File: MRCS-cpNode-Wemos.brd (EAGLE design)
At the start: 99.8 x 68.8 mm, 40 parts, among them CON1 3.5MM, CON2 3.5MM, J2 CONNECTOR-GROVE-4P-2.0-347013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, Q2 2n7002, Q3 2n7002, Q4 2n7002, Q5 2n7002, U3 NE555P, U4 MAX3465CPD

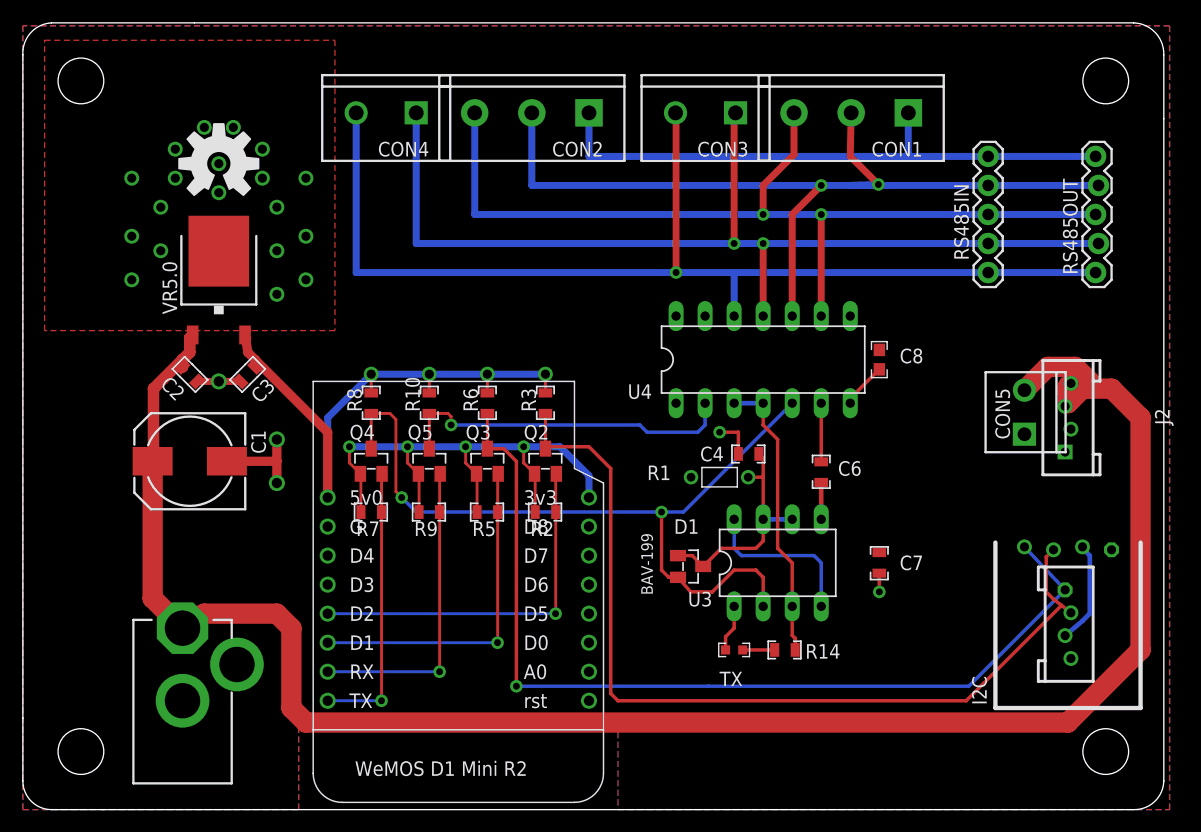
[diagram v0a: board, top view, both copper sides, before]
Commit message: 5.0
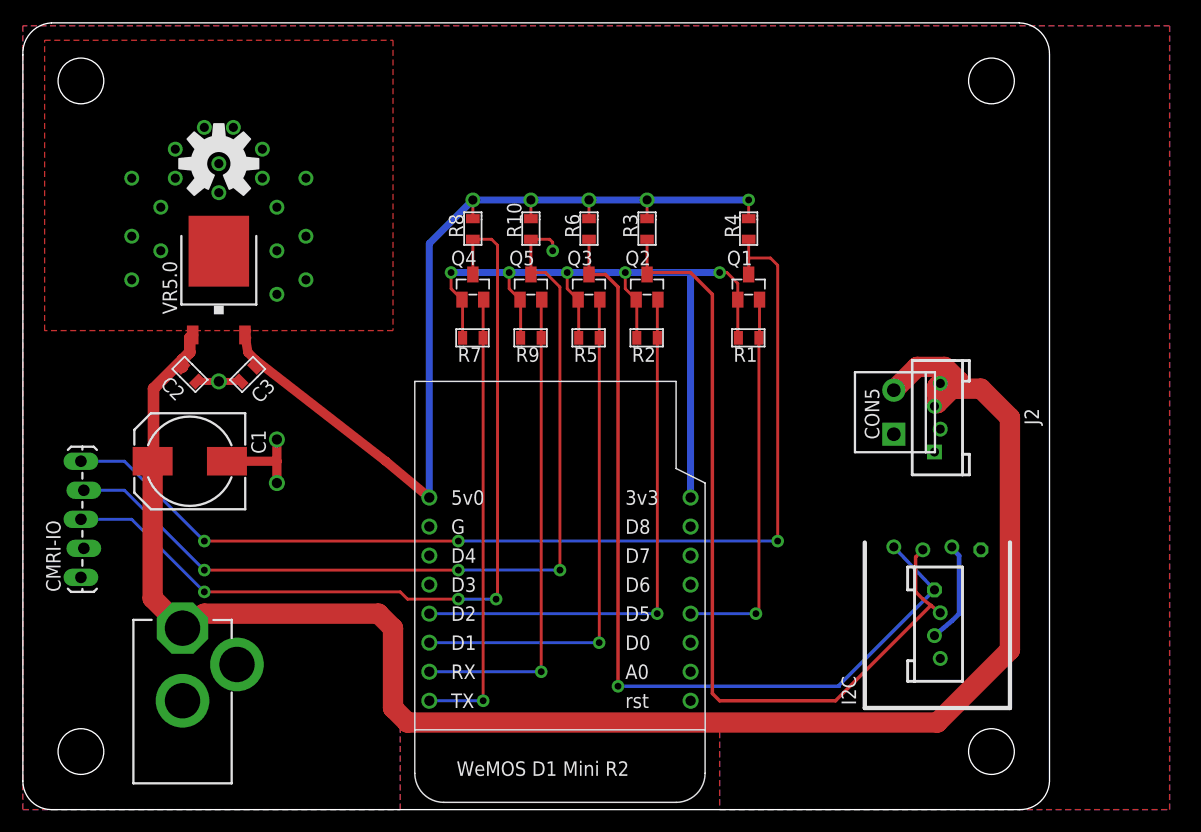
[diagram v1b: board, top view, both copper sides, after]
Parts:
- removed C4: 0.1uF, SPCoast:0805-CAP
- removed C6: .01uF, SPCoast:0805-CAP
- removed C7: .1uF, SPCoast:0805-CAP
- removed C8: .1uF, SPCoast:0603-CAP
- removed CON1, CON2: 3.5MM, SPCoast:SCREWTERMINAL-5MM-3
- removed CON3, CON4: (no value), SPCoast:SCREWTERMINAL-5MM-2
- removed D1: BAV-199, SPCoast:SOT23
- removed R14: 1k0, SPCoast:0805-RES
- removed RS485IN: (no value), SparkFun:1X05
- removed RS485OUT: (no value), SparkFun:1X05_LOCK
- removed TX: TX, SPCoast:0603-LED
- removed U3: NE555P, SparkFun:DIL-08
- removed U4: MAX3465CPD, maxim:DIL14
- added CMRI-IO: (no value), SPCoast:1X05_LOCK_LONGPADS
- added Q1: 2n7002, SPCoast:SOT23
- added R4: 10k, SPCoast:0805-RES
- BOARD: device SPCoast:BOARD-DINRAIL-2.7IN -> SPCoast:BOARD-DINRAIL-2.7IN-9CM
- C2, C3: device SPCoast:0805-CAP@1 -> SPCoast:0805-CAP
- R1: value (none) -> 10k; device SPCoast:1/6W-RES -> SPCoast:0805-RES
- moved Q2 17.6 mm to (54.6, 45.7)
- moved Q3 17.6 mm to (49.5, 45.7)
- moved Q4 17.6 mm to (39.4, 45.7)
- moved Q5 17.6 mm to (44.5, 45.7)
- moved R10 17.6 mm to (44.5, 50.8)
- moved R2 17.6 mm to (54.6, 41.3)
- moved R3 17.6 mm to (54.6, 50.8)
- moved R5 17.6 mm to (49.5, 41.3)
- moved R6 17.6 mm to (49.5, 50.8)
- moved R7 17.6 mm to (39.4, 41.3)
- moved R9 17.6 mm to (44.5, 41.3)
- moved R8 17.6 mm to (39.4, 50.8)
- moved R1 12.5 mm to (63.5, 41.3)
- moved CON5 11.4 mm to (76.2, 33.0)
- moved I2C 11.4 mm to (80.0, 22.9)
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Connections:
- removed net IN+: CON3.2, CON4.2, RS485IN.1, RS485OUT.1, U4.12
- removed net IN-: CON3.1, CON4.1, RS485IN.2, RS485OUT.2, U4.11
- removed net N$1: C4.1, D1.1, D1.3, R1.1, U3.6, U3.7
- removed net N$29: R14.2, TX.A
- removed net N$38: C6.1, U3.5
- removed net OUT+: CON1.3, CON2.3, RS485IN.3, RS485OUT.3, U4.9
- removed net OUT-: CON1.2, CON2.2, RS485IN.4, RS485OUT.4, U4.10
- removed net SHIELD: CON1.1, CON2.1, RS485IN.5, RS485OUT.5
- new net VCC: CMRI-IO.2
- net +3V3: now also Q1.1, R1.2
- net D5: now also Q1.2, R1.1
- net GND: now also CMRI-IO.1; no longer C4.2, C6.2, C7.2, C8.2, TX.C, U3.1, U4.6, U4.7
- net RXH: now also CMRI-IO.4; no longer U4.2
- net TXEN: now also CMRI-IO.5, Q1.3, R4.1; no longer R14.1, U3.3, U4.3, U4.4
- net TXH: now also CMRI-IO.3; no longer D1.2, U3.2, U4.5
- net VCCIO: now also R4.2; no longer C7.1, C8.1, R1.2, U3.4, U3.8, U4.14
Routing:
- net IN+: track 96.5 -> 0.00 mm, vias 1 -> 0
- net IN-: track 89.0 -> 0.00 mm, vias 2 -> 0
- net OUT+: track 82.1 -> 0.00 mm, vias 2 -> 0
- net OUT-: track 78.2 -> 0.00 mm, vias 2 -> 0
- net TXEN: track 25.3 -> 93.9 mm, vias 0 -> 3
- net SHIELD: track 51.9 -> 0.00 mm
- net RXH: track 30.5 -> 78.3 mm, vias 1 -> 4
- net D5: track 0.00 -> 33.3 mm, vias 0 -> 1
- net +3V3: track 48.4 -> 74.5 mm, vias 4 -> 5
- net N$1: track 20.4 -> 0.00 mm
- net GND: track 30.4 -> 12.0 mm, vias 24 -> 22
- net VCCIO: track 76.3 -> 92.3 mm, vias 4 -> 5
- net TX: track 24.6 -> 39.8 mm
- net SDA: track 32.2 -> 47.4 mm
- net RX: track 27.1 -> 42.4 mm
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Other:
- board size 99.8 x 68.8 mm -> 89.8 x 68.8 mm
- board text removed: "4-wire"
- board text removed: "AutoRTS"
- board text removed: "C/MRI Interface"
- board text removed: "IN"
- board text removed: "IN+"
- board text removed: "IN-"
- board text removed: "OUT"
- board text removed: "Out+"
- board text removed: "Out-"
- board text removed: "RS-485"
- board text removed: "RX"
- board text removed: "Shield"
- board text removed: "TX"
